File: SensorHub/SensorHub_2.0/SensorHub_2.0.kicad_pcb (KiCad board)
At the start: 4 copper layers, 30 x 28 mm, 59 parts, among them J1 USB_C_Receptacle, J2 658561423020, J3 658561423020, J4 USB_C_Receptacle, J5 FTSH-105-01-L-DV-K-A, U1 R7FA4E2B93CFM#AA0, U2 MYRGM080200C41RA, U3 TCAN334, U4 USBLC6-4SC6, U6 LSM6DSM, Y1 ASH7KW-32.768KHZ-L-T

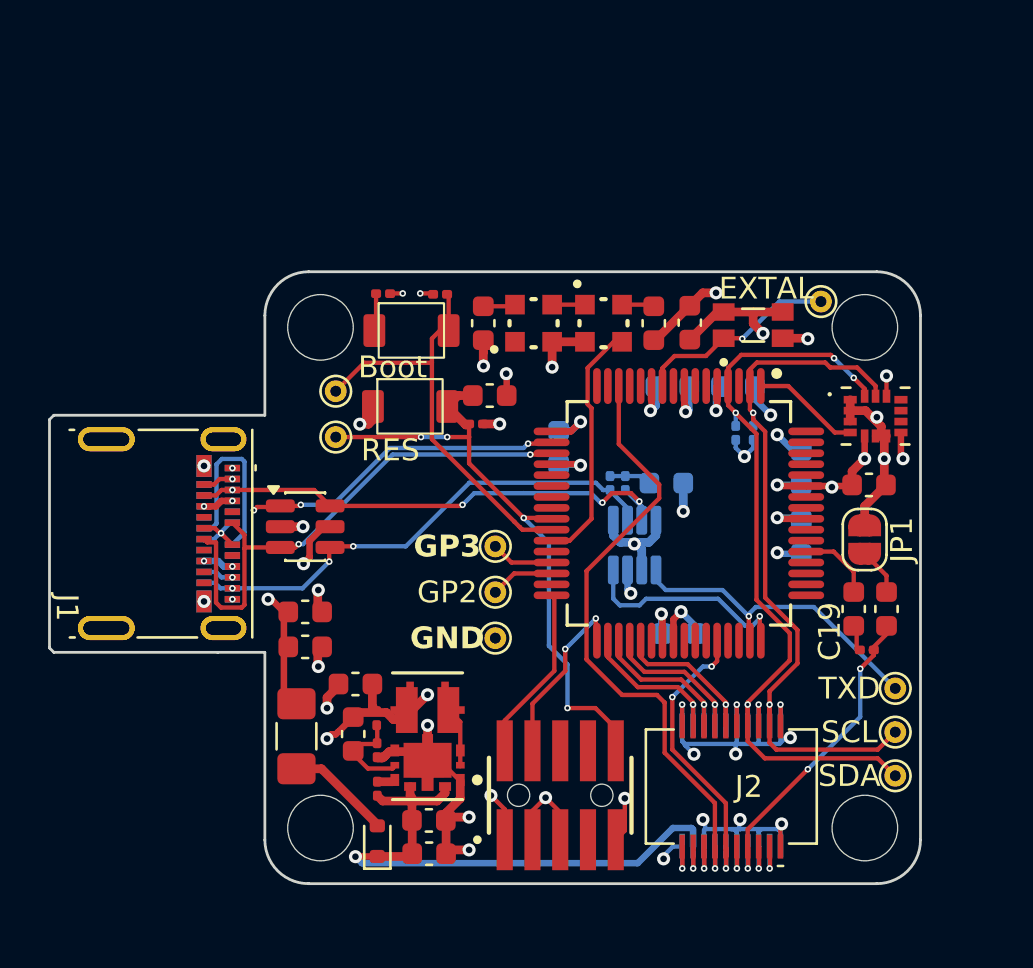
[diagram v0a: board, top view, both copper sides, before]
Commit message: Vesrion 2
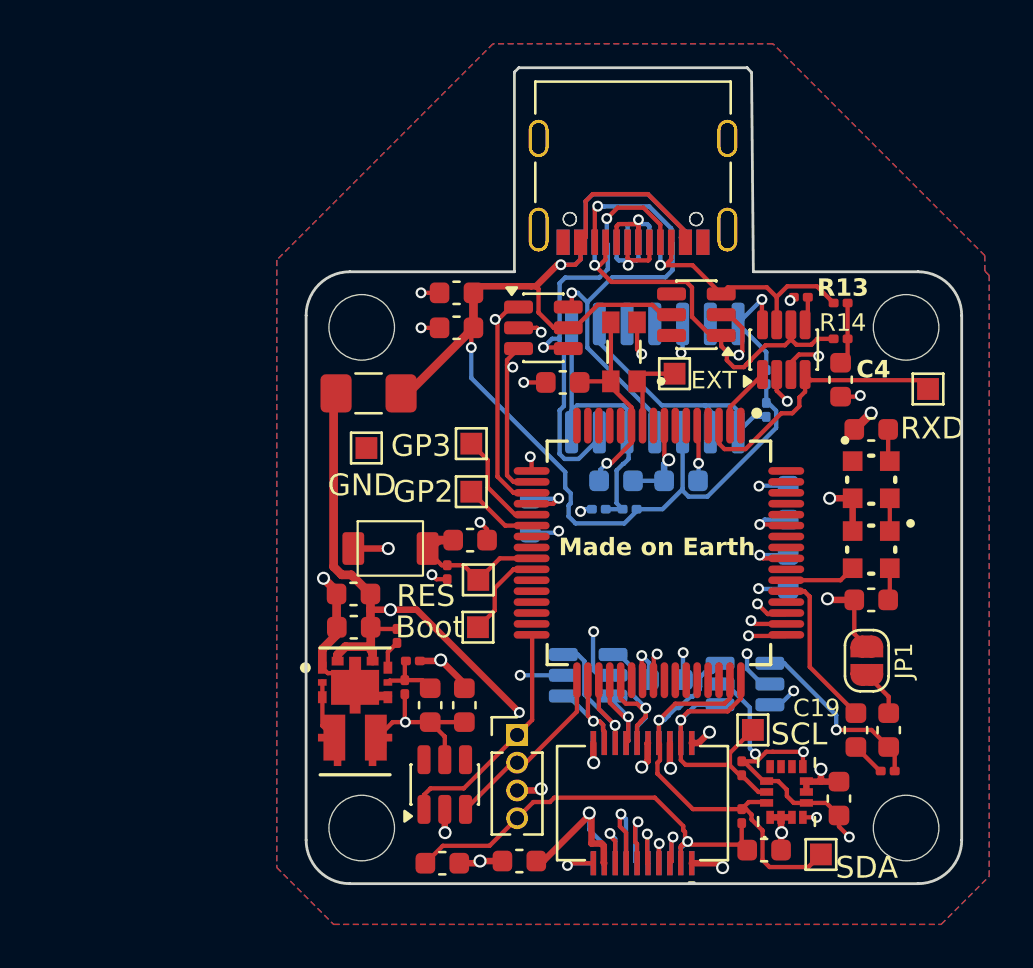
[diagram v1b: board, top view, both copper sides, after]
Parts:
- removed the Boot at (144.9, 73.5)
- removed the Boot at (141.4, 76.3)
- removed D3: 1N4148WT, Diode_SMD:D_SOD-523
- removed EXTAL, TXD: TestPoint, TestPoint:TestPoint_THTPad_D1.0mm_Drill0.5mm
- removed the GND at (148.7, 87.6)
- removed J4: USB_C_Receptacle, Connector_USB:USB_C_Receptacle_Molex_105450-0101
- removed J5: FTSH-105-01-L-DV-K-A, FTSH-105-01-L-DV-K-A:SAMTEC_FTSH-105-01-L-DV-K-A
- removed R5: 1.5 K, Resistor_SMD:R_0201_0603Metric
- removed R6: 10 K, Resistor_SMD:R_0201_0603Metric
- removed the RES at (141.4, 78.4)
- removed the SCL at (167.0, 91.9)
- removed the SDA at (167.0, 93.9)
- added Boot: TestPoint, TestPoint:TestPoint_Pad_1.0x1.0mm, F.Cu at (147.9, 87.1)
- added C21: 0.1 uF, Capacitor_SMD:C_0603_1608Metric, F.Cu at (146.9, 73.4)
- added C22: 0.1 uF, Capacitor_SMD:C_0603_1608Metric, F.Cu at (146.3, 97.9)
- added C23: 0.1 uF, Capacitor_SMD:C_0603_1608Metric, F.Cu at (149.8, 97.8)
- added EXT: TestPoint, TestPoint:TestPoint_Pad_1.0x1.0mm, F.Cu at (156.9, 75.5)
- added GND: TestPoint, TestPoint:TestPoint_Pad_1.0x1.0mm, F.Cu at (142.8, 78.9)
- added J6: USB_C_Receptacle_USB2.0_16P, Connector_USB:USB_C_Receptacle_Palconn_UTC16-G, B.Cu at (155.0, 67.0)
- added J8: USB_C_Receptacle_USB2.0_16P, Connector_USB:USB_C_Receptacle_Palconn_UTC16-G, F.Cu at (155.0, 67.0)
- added R10: 5.1 K, Resistor_SMD:R_0201_0603Metric, B.Cu at (161.1, 75.7)
- added R16: 10k, Resistor_SMD:R_0201_0603Metric, F.Cu at (162.7, 72.0)
- added R3: 100 K, Resistor_SMD:R_0201_0603Metric, B.Cu at (154.8, 81.7)
- added R8: 5.1 K, Resistor_SMD:R_0201_0603Metric, B.Cu at (153.4, 81.7)
- added R9: 5.1 K, Resistor_SMD:R_0201_0603Metric, B.Cu at (161.1, 77.2)
- added RES: TestPoint, TestPoint:TestPoint_Pad_1.0x1.0mm, F.Cu at (147.9, 84.9)
- added RXD: TestPoint, TestPoint:TestPoint_Pad_1.0x1.0mm, F.Cu at (168.5, 76.2)
- added SCL: TestPoint, TestPoint:TestPoint_Pad_1.0x1.0mm, F.Cu at (160.5, 91.8)
- added SDA: TestPoint, TestPoint:TestPoint_Pad_1.0x1.0mm, F.Cu at (163.6, 97.5)
- added U10: LMV339, Package_SO:SOIC-14_3.9x8.7mm_P1.27mm, B.Cu at (156.0, 75.7)
- added U5: USBLC6-4SC6, Package_TO_SOT_SMD:SOT-23-6, B.Cu at (160.1, 89.7)
- added U7: USBLC6-4SC6, Package_TO_SOT_SMD:SOT-23-6, F.Cu at (157.9, 72.8)
- added U8: USBLC6-4SC6, Package_TO_SOT_SMD:SOT-23-6, B.Cu at (152.9, 89.3)
- added U9: USBLC6-4SC6, Package_TO_SOT_SMD:SOT-23-6, F.Cu at (146.4, 94.3)
- C4, R13, R14, R15, R7, U3: moved to F.Cu
- GP2, GP3: footprint TestPoint:TestPoint_THTPad_D1.0mm_Drill0.5mm -> TestPoint:TestPoint_Pad_1.0x1.0mm
- J1: value USB_C_Receptacle -> Conn_01x04_Pin; footprint Connector_USB:USB_C_Receptacle_Molex_105450-0101 -> Connector_PinHeader_1.27mm:PinHeader_1x04_P1.27mm_Vertical
- moved C5 23.0 mm to (161.0, 97.3)
- moved J1 18.7 mm to (149.7, 92.0), turned to 0 degrees
- moved C9 18.4 mm to (165.9, 78.0), turned to 180 degrees
- moved U6 17.7 mm to (162.0, 94.6), turned to 90 degrees
- moved R15 17.5 mm to (160.0, 95.7)
- moved D4 17.0 mm to (165.9, 80.3), turned to -90 degrees
- moved C20 16.2 mm to (146.9, 71.8), turned to 180 degrees
- moved C15 16.1 mm to (165.9, 85.8), turned to 180 degrees
- moved D5 16.0 mm to (165.9, 83.5), turned to 180 degrees
- moved F1 16.0 mm to (142.9, 76.4), turned to 0 degrees
- moved R7 15.4 mm to (160.0, 93.6), turned to -90 degrees
- moved C8 14.4 mm to (164.4, 94.9), turned to 90 degrees
- moved U4 14.2 mm to (150.9, 73.4)
- moved R13 12.8 mm to (164.5, 72.3), turned to 180 degrees
- moved R14 12.4 mm to (164.5, 73.9), turned to 180 degrees
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- renumbered RES to SW1
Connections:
- C5 pad 1: /V_Bus -> +3.3V
- F1 pad 1: Net-(D3-A) -> +5V
- J2 pad 2: /+3.3V -> +3.3V
- J3 pad 12: /+3.3V -> +3.3V
- U1 pad 1: /INT1 -> unconnected-(U1-P400-Pad1)
- U1 pad 14: /GP1 -> unconnected-(U1-P409-Pad14)
- U1 pad 2: /SCL_0 -> /TXD
- U1 pad 21: unconnected-(U1-CACREF-Pad21) -> /GP3
- U1 pad 22: unconnected-(U1-P206-Pad22) -> /GP2
- U1 pad 27: /RA4E2_microcontroller/LED -> unconnected-(U1-P200-Pad27)
- U1 pad 29: /GP3 -> unconnected-(U1-P303-Pad29)
- U1 pad 3: unconnected-(U1-CACREF-Pad3) -> /RXD
- U1 pad 30: /GP2 -> unconnected-(U1-P302-Pad30)
- U1 pad 4: /SDA_0 -> unconnected-(U1-P403-Pad4)
- U1 pad 44: /INT2 -> unconnected-(U1-P104-Pad44)
- U1 pad 47: /TXD -> /SDA_0
- U1 pad 48: /RXD -> /SCL_0
- U1 pad 49: unconnected-(U1-CACREF-Pad49) -> /GP1
- U1 pad 50: unconnected-(U1-P008-Pad50) -> /INT2
- U1 pad 51: unconnected-(U1-P006-Pad51) -> /INT1
- U1 pad 54: unconnected-(U1-P013-Pad54) -> /RA4E2_microcontroller/LED
- U3 pad 5: GND -> Net-(U3-SHDN)
- U3 pad 8: GND -> /EN
- U4 pad 1: /USB_DM -> /USB_DP
- U4 pad 3: /USB_DP -> /USB_DM
- U4 pad 4: /Can_L -> /USB_C_2.0+SBUS/CC1
- U4 pad 6: /Can_H -> /USB_C_2.0+SBUS/CC2
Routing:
- net /V_Bus: track 18.5 -> 66.1 mm, vias 6 -> 2
- net +3.3V: track 39.4 -> 68.9 mm, vias 17 -> 13
- net /RES: track 28.6 -> 7.09 mm, vias 4 -> 0
- net /USB_C_2.0+SBUS/CC1: track 0.00 -> 21.3 mm, vias 0 -> 2
- net /USB_C_2.0+SBUS/CC2: track 0.00 -> 20.8 mm, vias 0 -> 2
- net GND: track 97.8 -> 79.1 mm, vias 45 -> 41
- net /SCL_0: track 34.1 -> 15.6 mm, vias 2 -> 1
- net /Can_H: track 29.1 -> 13.0 mm, vias 5 -> 1
- net /RA4E2_microcontroller/Boot: track 19.5 -> 4.15 mm
- net Net-(U10A-+): track 0.00 -> 14.4 mm
- net +5V: track 28.2 -> 41.2 mm, vias 2 -> 3
- net /SDA_0: track 36.5 -> 24.0 mm, vias 4 -> 1
- net Net-(U10D-+): track 0.00 -> 12.4 mm
- net /Can_L: track 30.4 -> 18.1 mm, vias 4 -> 1
- net /TXD: track 15.0 -> 2.95 mm, vias 1 -> 0
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- added copper zone on B.Cu, net GND
- added copper zone on F.Cu, net GND
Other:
- board size 30 x 28 mm -> 30 x 37.3 mm
- board text added: "CAN Pull-Up R13,R14,C4 (optional)"
- board text removed: "0.5\.1"
- board text removed: "0.6\.1"
- board text removed: "0.6\.15"
- board text removed: "0.8\.15"
